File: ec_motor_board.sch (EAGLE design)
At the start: 26 parts

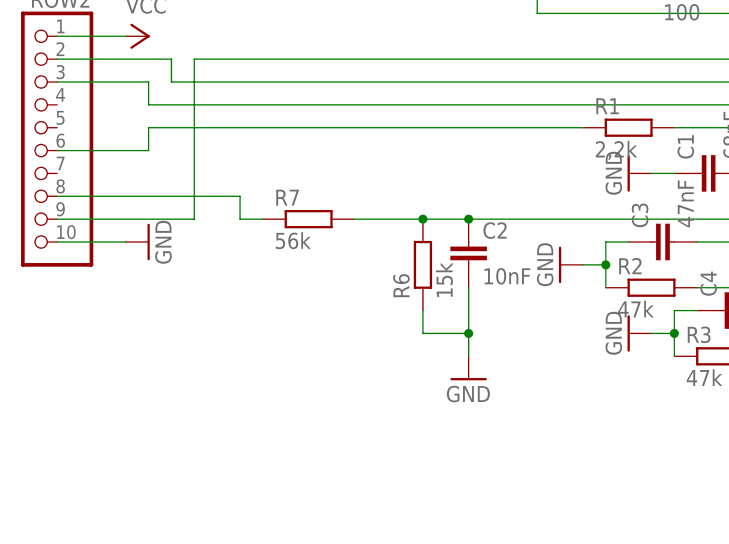
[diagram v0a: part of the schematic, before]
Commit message: ec_motor_board: added an 0 ohm resistor which can connect vref to vcc to disable power regulation
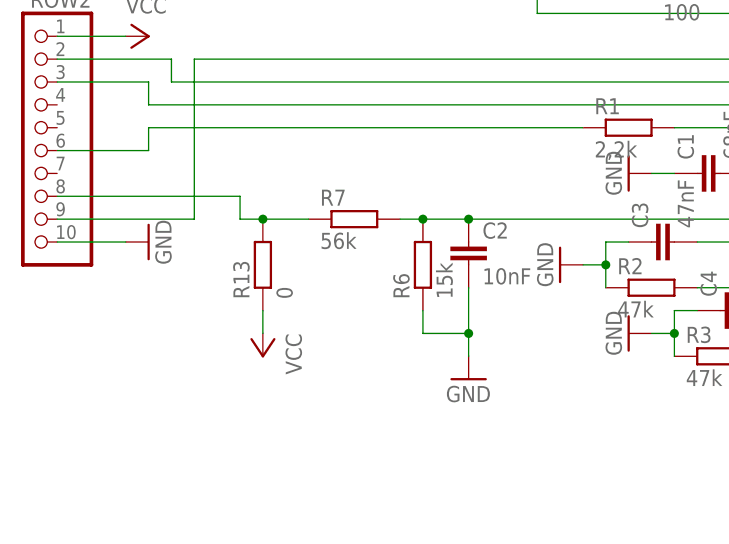
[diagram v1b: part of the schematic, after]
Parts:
- added R13: 0, resistor:R-EU_R1206
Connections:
- net N$14: now also R13.2
- net VCC: now also R13.1
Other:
- moved on the sheet: R7
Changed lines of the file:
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@@
 <part name="R12" library="resistor" deviceset="R-EU_" device="R1206"/>
 <part name="P+7" library="supply1" deviceset="VCC" device=""/>
+<part name="R13" library="resistor" deviceset="R-EU_" device="R1206" value="0"/>
+<part name="P+8" library="supply1" deviceset="VCC" device=""/>
 </parts>
 <sheets>
@@
 <instance part="D2" gate="G$1" x="-27.94" y="30.48" rot="R180"/>
 <instance part="R6" gate="G$1" x="-55.88" y="-12.7" rot="R90"/>
-<instance part="R7" gate="G$1" x="-68.58" y="-7.62"/>
+<instance part="R7" gate="G$1" x="-63.5" y="-7.62"/>
 <instance part="R8" gate="G$1" x="33.02" y="-12.7"/>
 <instance part="R9" gate="G$1" x="33.02" y="-10.16"/>
@@
 <instance part="R12" gate="G$1" x="33.02" y="-7.62" rot="R180"/>
 <instance part="P+7" gate="VCC" x="43.18" y="-7.62" rot="R270"/>
+<instance part="R13" gate="G$1" x="-73.66" y="-12.7" rot="R90"/>
+<instance part="P+8" gate="VCC" x="-73.66" y="-22.86" rot="R180"/>
 </instances>
 <busses>
@@
 <pinref part="R6" gate="G$1" pin="2"/>
 <junction x="-55.88" y="-7.62"/>
-<wire x1="-55.88" y1="-7.62" x2="-63.5" y2="-7.62" width="0.1524" layer="91"/>
+<wire x1="-55.88" y1="-7.62" x2="-58.42" y2="-7.62" width="0.1524" layer="91"/>
 <pinref part="R7" gate="G$1" pin="2"/>
 </segment>
@@
 <segment>
 <pinref part="R7" gate="G$1" pin="1"/>
+<wire x1="-68.58" y1="-7.62" x2="-73.66" y2="-7.62" width="0.1524" layer="91"/>
 <wire x1="-73.66" y1="-7.62" x2="-76.2" y2="-7.62" width="0.1524" layer="91"/>
 <wire x1="-76.2" y1="-7.62" x2="-76.2" y2="-5.08" width="0.1524" layer="91"/>
 <pinref part="ROW2" gate="A" pin="8"/>
 <wire x1="-76.2" y1="-5.08" x2="-96.52" y2="-5.08" width="0.1524" layer="91"/>
+<pinref part="R13" gate="G$1" pin="2"/>
+<junction x="-73.66" y="-7.62"/>
 </segment>
 </net>
@@
 <wire x1="40.64" y1="-7.62" x2="38.1" y2="-7.62" width="0.1524" layer="91"/>
 </segment>
-</net>
+<segment>
+<pinref part="R13" gate="G$1" pin="1"/>
+<pinref part="P+8" gate="VCC" pin="VCC"/>
+<wire x1="-73.66" y1="-20.32" x2="-73.66" y2="-17.78" width="0.1524" layer="91"/>
+</segment>
+</net>
